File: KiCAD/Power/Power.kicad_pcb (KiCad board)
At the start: 2 copper layers, 65 x 60 mm, 18 parts, among them J1 Barrel_Jack_Switch_MountingPin, J2 Conn_01x03_Pin, U1 LM317 TO-220, U2 LM337 TO-220, U3 LM336Z-2.5v

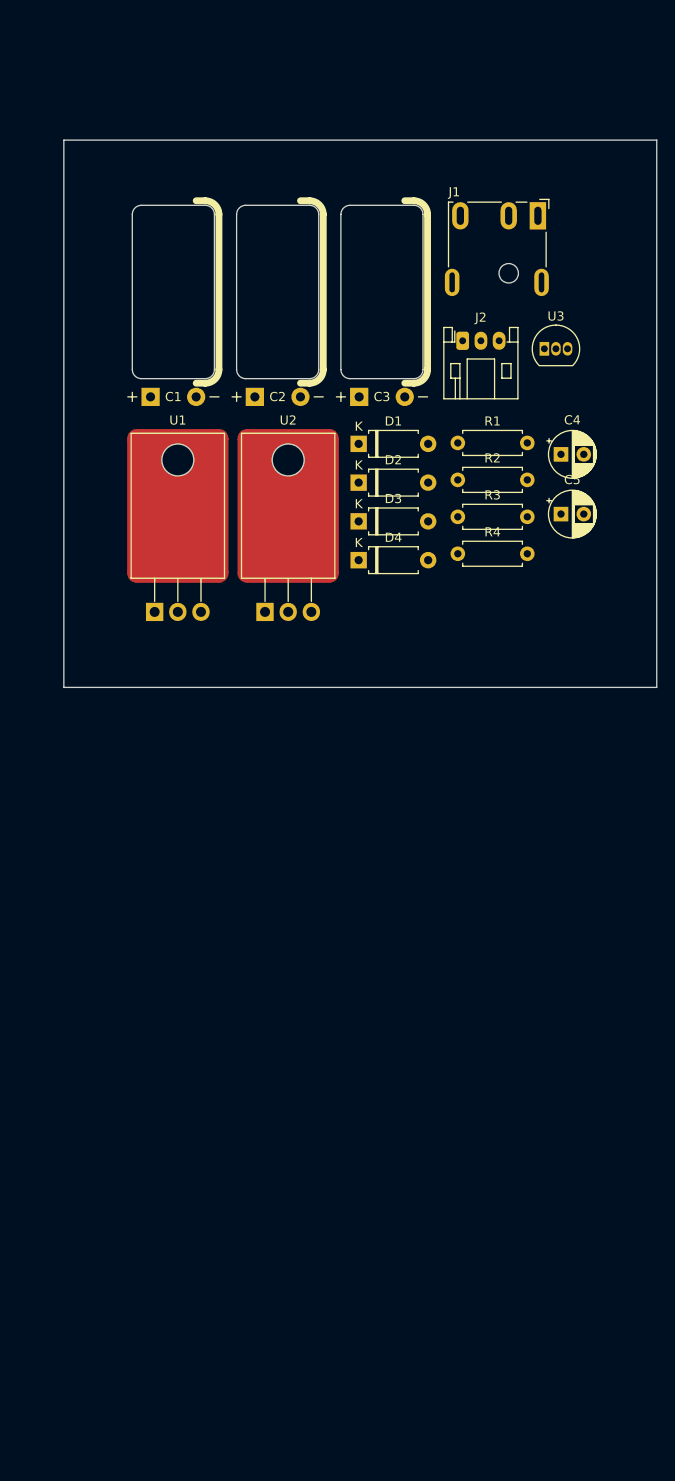
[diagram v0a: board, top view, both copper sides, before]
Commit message: Power PCB
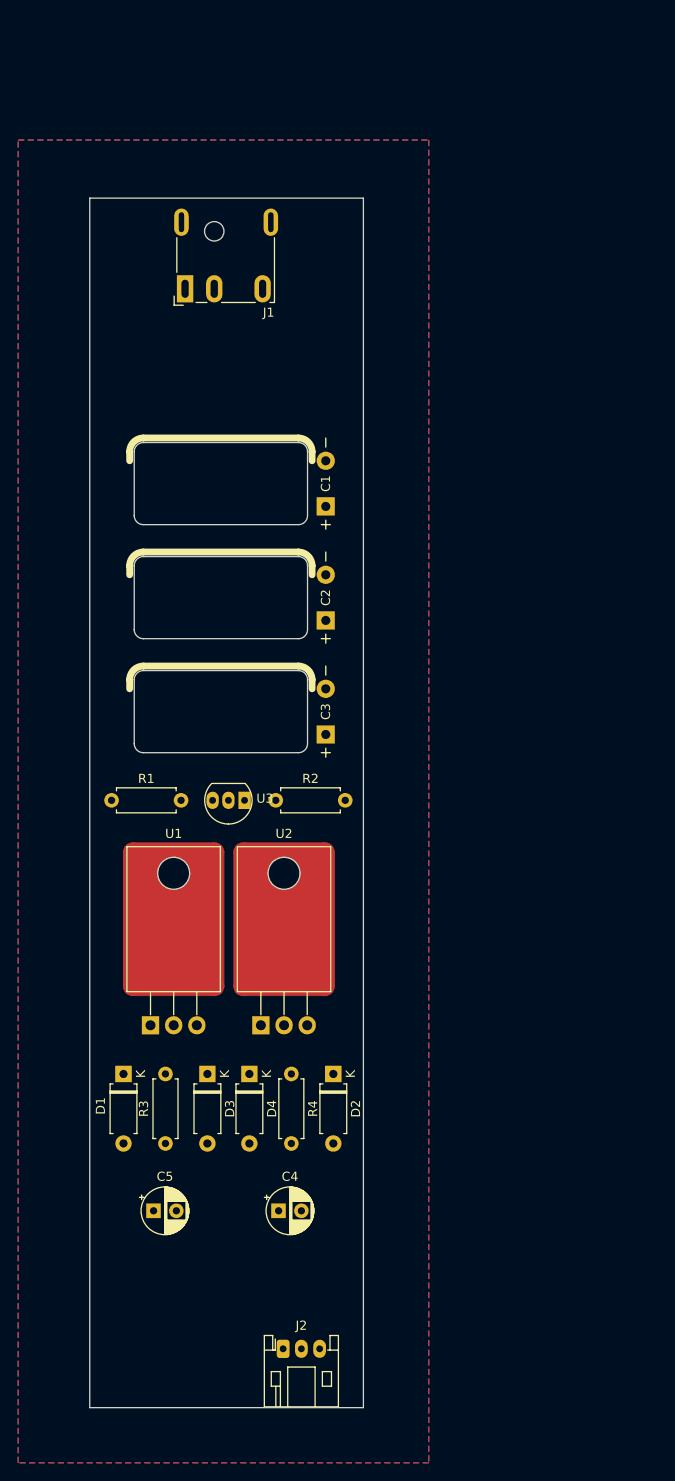
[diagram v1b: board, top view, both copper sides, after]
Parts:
- U3: footprint Package_TO_SOT_THT:TO-92_Inline -> HackSynth:TO-92_Inline - Handsolder
- moved J2 112.2 mm to (109.0, 162.5)
- moved C4 88.5 mm to (108.5, 147.4)
- moved C5 88.5 mm to (94.8, 147.4)
- moved R3 75.8 mm to (96.1, 140.0), turned to 90 degrees
- moved D1 73.7 mm to (91.5, 132.4), turned to -90 degrees
- moved D2 64.9 mm to (114.5, 132.4), turned to -90 degrees
- moved D3 62.8 mm to (100.7, 132.4), turned to -90 degrees
- moved R4 59.9 mm to (109.9, 132.4), turned to -90 degrees
- moved U3 59.7 mm to (104.3, 102.4), turned to 180 degrees
- moved D4 57.6 mm to (105.3, 132.4), turned to -90 degrees
- moved R1 54.6 mm to (90.2, 102.4)
- moved U1 45.3 mm to (97.0, 127.0)
- moved U2 45.3 mm to (109.1, 127.0)
- moved R2 40.4 mm to (108.2, 102.4)
- moved J1 39.5 mm to (98.3, 46.3), turned to 180 degrees
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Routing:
- added copper zone on B.Cu, net GND
- added copper zone on F.Cu, net GND
- added copper zone on In1.Cu, net GND
- added copper zone on In2.Cu, net GND
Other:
- board size 65 x 60 mm -> 30 x 132.6 mm
- copper layers 2 -> 4

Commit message: Power PCB
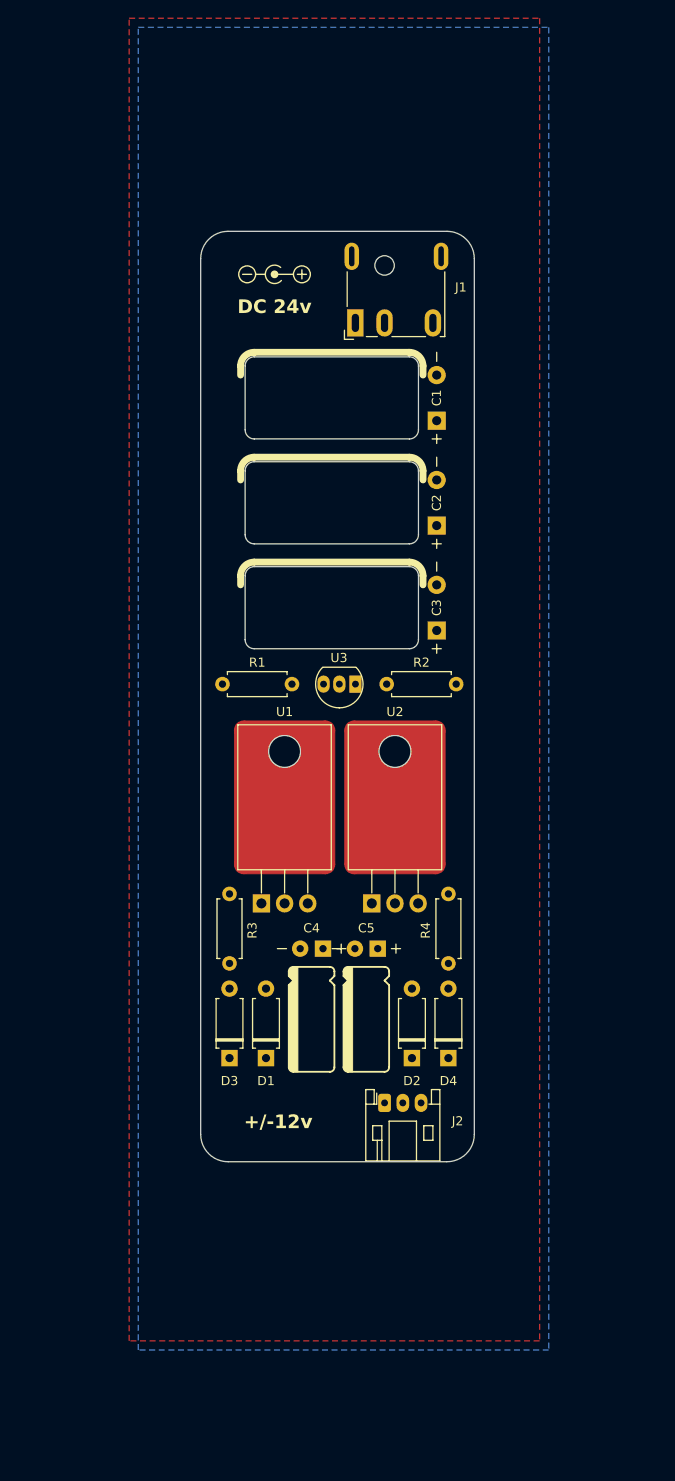
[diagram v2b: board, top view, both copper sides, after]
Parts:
- added G***: LOGO, CCHS:PancakeLegend_Logo_SolderMask, B.Cu at (115.2, 126.5)
- added REF**: Symbol_Barrel_Polarity, Symbol:Symbol_Barrel_Polarity, F.Cu at (108.1, 44.6)
- added REF**: CCHS_Logo_Small_NoText, CCHS:CCHS_Logo_Small_NoText, B.Cu at (107.8, 53.0)
- C4, C5: footprint Capacitor_THT:CP_Radial_D5.0mm_P2.50mm -> HackSynth:CP_Radial_D5.2mm_P2.50mm_LayDown
- moved C5 37.0 mm to (118.2, 118.6), turned to 180 degrees
- moved J2 29.2 mm to (120.2, 135.6)
- moved C4 29.0 mm to (112.2, 118.6), turned to 180 degrees
- moved R4 26.2 mm to (127.2, 112.6)
- moved D4 21.9 mm to (127.2, 130.6), turned to 90 degrees
- moved R3 21.0 mm to (103.2, 120.3)
- moved J1 19.0 mm to (117.0, 50.0)
- moved U2 18.1 mm to (121.3, 113.7)
- moved U1 18.1 mm to (109.2, 113.7)
- moved R1 17.6 mm to (102.4, 89.6)
- moved R2 17.6 mm to (120.4, 89.6)
- moved U3 17.6 mm to (116.5, 89.6)
- moved C3 16.7 mm to (125.9, 83.8)
- moved C2 16.0 mm to (125.9, 72.3)
- moved D1 15.7 mm to (107.2, 130.6), turned to 90 degrees
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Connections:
- net Net-(D3-K) renamed VDD
- net Net-(D4-A) renamed VSS
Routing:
- net Net-(D2-A): track 0.00 -> 62.8 mm
- net Net-(D2-K): track 0.00 -> 22.1 mm
- net Net-(D1-A): track 0.00 -> 17.3 mm
- added copper zone on In2.Cu, net Net-(D1-K)
- added copper zone on F.Cu, net VDD
- added copper zone on B.Cu, net VSS
- removed copper zone on B.Cu, net GND
- removed copper zone on F.Cu, net GND
- removed copper zone on In2.Cu, net GND
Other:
- board size 30 x 132.6 mm -> 30 x 102 mm
- board text added: "+/-12v"
- board text added: "DC 24v"
- board text added: "POWER v1-0"
